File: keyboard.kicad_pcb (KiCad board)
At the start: 2 copper layers, 129.8 x 72.4 mm, 119 parts, among them P1 USB_B, P10 CONN_01X01, P2 CONN_02X03, P3 CONN_01X01, P4 CONN_01X01, P5 CONN_01X01, P6 CONN_01X01, P7 CONN_01X01, P8 CONN_01X01, P9 CONN_01X01, SW10 SW_PUSH, SW11 SW_PUSH, SW12 SW_PUSH, SW13 SW_PUSH, SW14 SW_PUSH, SW15 SW_PUSH, SW2 SW_PUSH, SW24 SW_PUSH, SW25 SW_PUSH, SW26 SW_PUSH, SW27 SW_PUSH, SW28 SW_PUSH, SW29 SW_PUSH, SW3 SW_PUSH, SW30 SW_PUSH, SW31 SW_PUSH, SW32 SW_PUSH, SW33 SW_PUSH, SW34 SW_PUSH, SW35 SW_PUSH, SW36 SW_PUSH, SW37 SW_PUSH, SW4 SW_PUSH, SW5 SW_PUSH, SW6 SW_PUSH, SW7 SW_PUSH, SW8 SW_PUSH, SW9 SW_PUSH, U1 ATmega32U4, X1 CRYSTAL_SMD

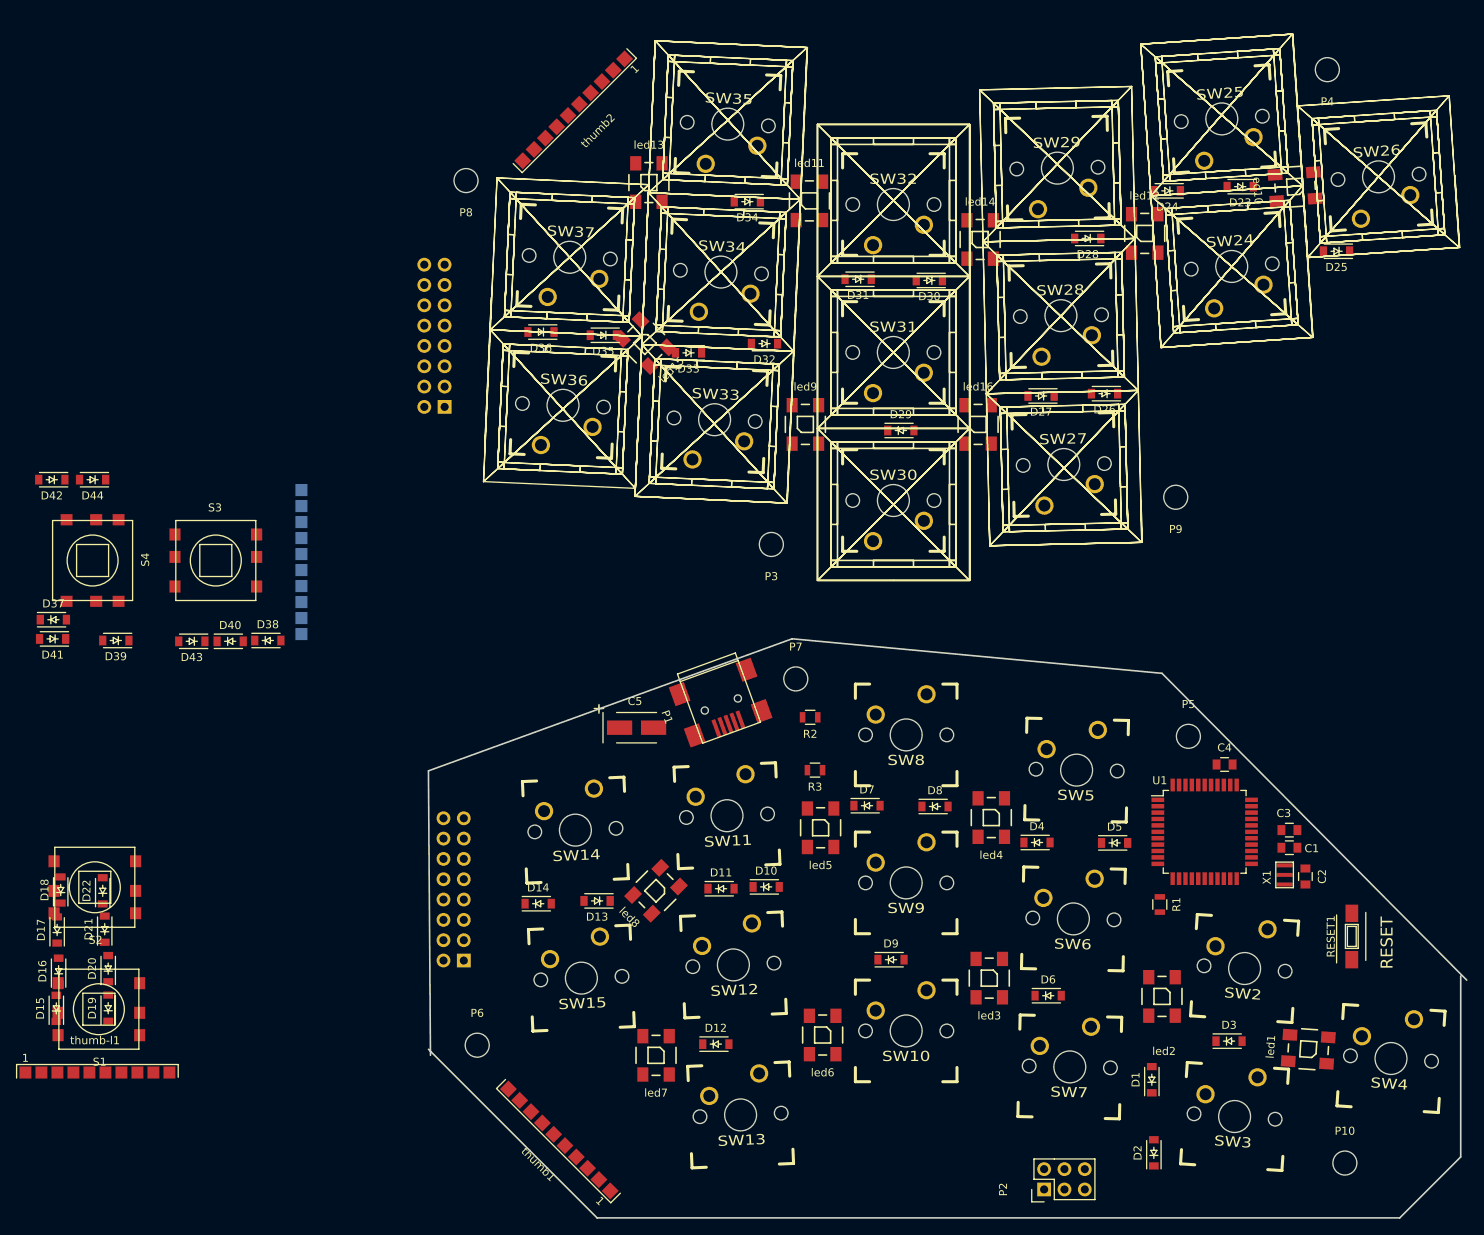
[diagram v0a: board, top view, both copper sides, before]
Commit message: nearly routed
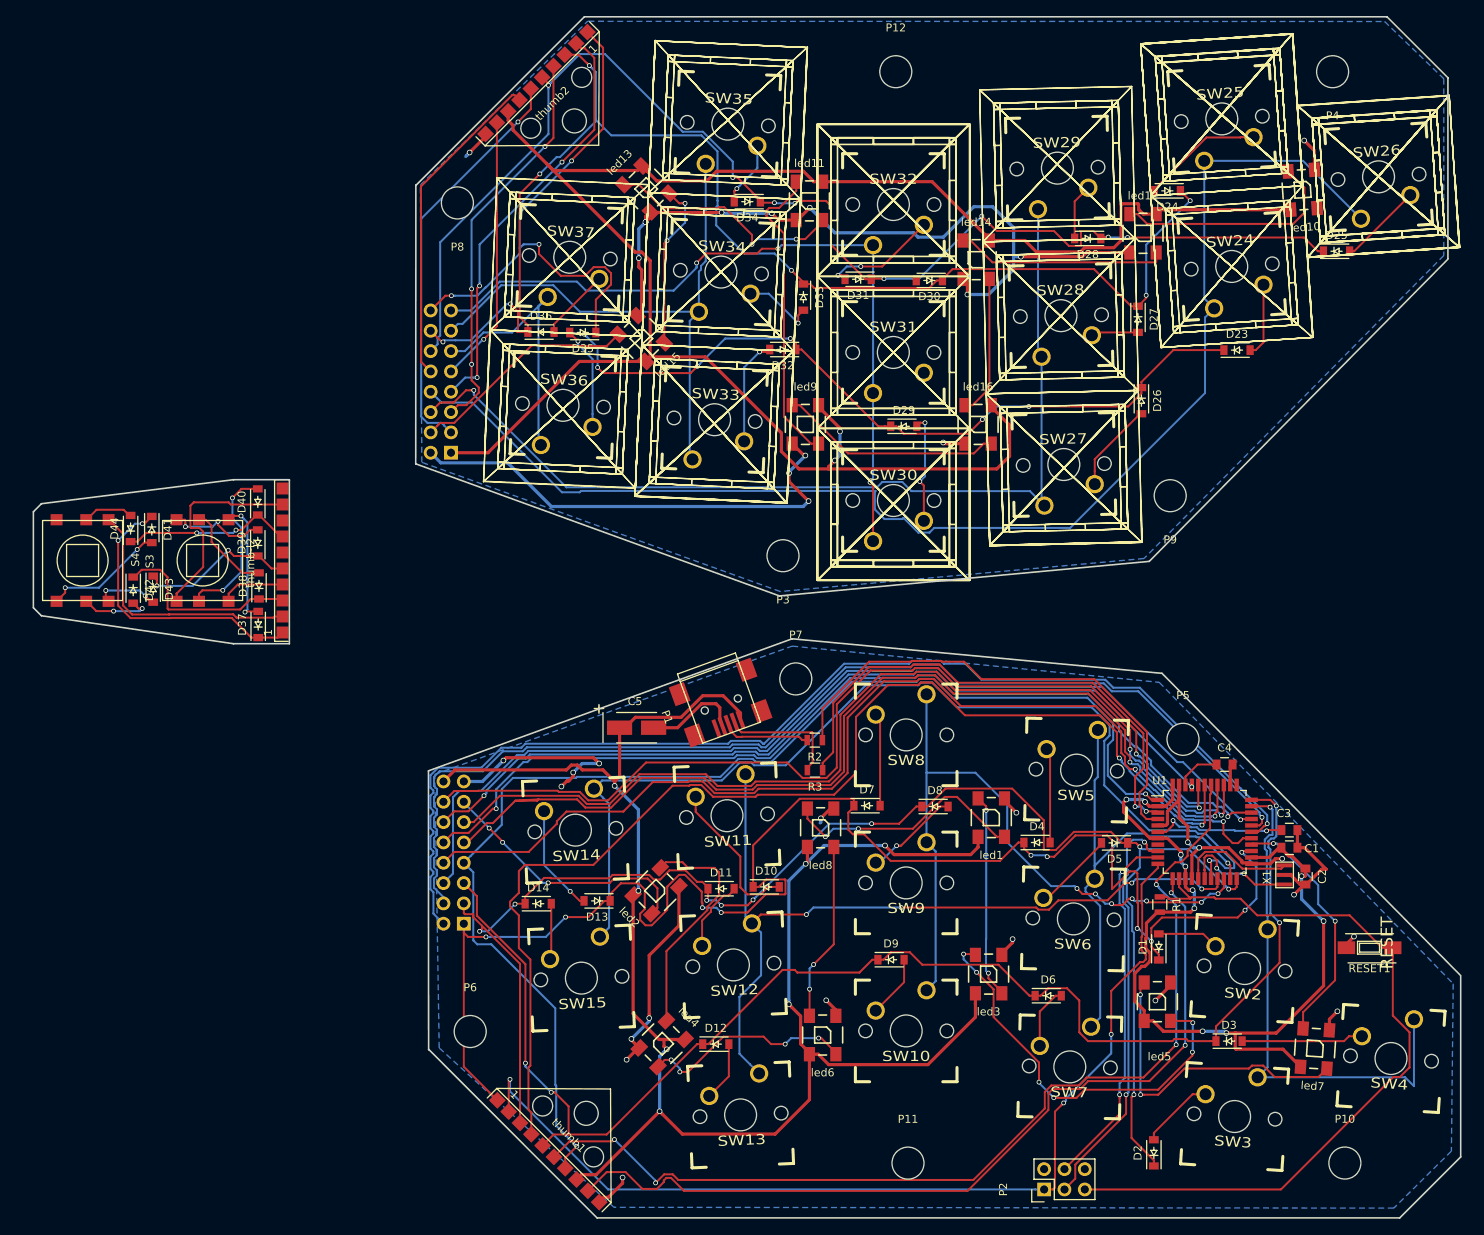
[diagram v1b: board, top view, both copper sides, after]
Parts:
- removed D15, D16, D17, D18, D19, D20, D21, D22: D, Diodes_SMD:SOD-123
- removed S1, S2: alps_4way, fp:alps 4way smt
- removed thumb-l1: CONN_02X05, fp:thumbpad connector
- added P11: CONN_01X01, Mounting_Holes:MountingHole_4mm, F.Cu at (148.8, 165.9)
- added P12: CONN_01X01, Mounting_Holes:MountingHole_4mm, F.Cu at (147.3, 29.5)
- P10, P3, P4, P5, P6, P7, P8, P9: footprint Mounting_Holes:MountingHole_3mm -> Mounting_Holes:MountingHole_4mm
- thumb-l2: moved to F.Cu
- moved conn1 64.6 mm to (93.3, 136.0)
- moved conn2 63.5 mm to (91.7, 77.1)
- moved D37 25.6 mm to (67.6, 98.6), turned to 90 degrees
- moved D39 21.5 mm to (67.5, 88.4), turned to 90 degrees
- moved D23 20.4 mm to (189.9, 64.3), turned to 0 degrees
- moved D41 18.5 mm to (54.3, 86.7), turned to 270 degrees
- moved thumb1 18.1 mm to (97.5, 158.1), turned to 315 degrees
- moved thumb-l2 18.0 mm to (70.7, 99.6), turned to 90 degrees
- moved D40 17.8 mm to (67.5, 83.3), turned to 90 degrees
- moved D42 17.1 mm to (52.0, 94.3), turned to 270 degrees
- moved D1 16.6 mm to (180.2, 138.9)
- moved D33 16.0 mm to (135.8, 57.7), turned to 270 degrees
- moved D27 15.4 mm to (177.6, 60.5), turned to 270 degrees
- moved D43 8.12 mm to (54.5, 94.2), turned to 270 degrees
- moved D44 7.73 mm to (51.6, 86.6), turned to 90 degrees
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- renumbered led4 to led1, led8 to led2, led7 to led4, led2 to led5, led1 to led7, led5 to led8
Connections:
- D1 pad 1: /left keys/row1 -> /right keys/row1
- D10 pad 1: /left keys/row1 -> /right keys/row1
- D11 pad 1: /left keys/row2 -> /right keys/row2
- D12 pad 1: /left keys/row3 -> /right keys/row3
- D13 pad 1: /left keys/row1 -> /right keys/row1
- D14 pad 1: /left keys/row2 -> /right keys/row2
- D2 pad 1: /left keys/row2 -> /right keys/row2
- D3 pad 1: /left keys/row3 -> /right keys/row3
- D37 pad 1: /left keys/row1 -> /left keys/thumb/row1
- D38 pad 1: /left keys/row2 -> /left keys/thumb/row2
- D39 pad 1: /left keys/row3 -> /left keys/thumb/row3
- D4 pad 1: /left keys/row1 -> /right keys/row1
- D40 pad 1: /left keys/row4 -> /left keys/thumb/row4
- D41 pad 1: /left keys/row1 -> /left keys/thumb/row1
- D42 pad 1: /left keys/row2 -> /left keys/thumb/row2
- D43 pad 1: /left keys/row3 -> /left keys/thumb/row3
- D44 pad 1: /left keys/row4 -> /left keys/thumb/row4
- D5 pad 1: /left keys/row2 -> /right keys/row2
- D6 pad 1: /left keys/row3 -> /right keys/row3
- D7 pad 1: /left keys/row1 -> /right keys/row1
- D8 pad 1: /left keys/row2 -> /right keys/row2
- D9 pad 1: /left keys/row3 -> /right keys/row3
- S3 pad 4: /left keys/col6 -> /left keys/thumb/col1
- S4 pad 4: /left keys/col7 -> /left keys/thumb/col2
- U1 pad 1: /left keys/row4 -> /right keys/row4
- U1 pad 22: /left keys/row2 -> /right keys/row2
- U1 pad 25: /left keys/row1 -> /right keys/row1
- U1 pad 27: /left keys/col6 -> /col6
- U1 pad 28: /left keys/col3 -> /col3
- U1 pad 29: /left keys/col4 -> /col4
- U1 pad 30: /left keys/col5 -> /col5
- U1 pad 31: /left keys/col7 -> /col7
- U1 pad 33: /left keys/row3 -> /right keys/row3
- U1 pad 36: /left keys/col2 -> /col2
- U1 pad 37: /left keys/col1 -> /col1
- U1 pad 40: /left keys/joy-y -> /l-joy-y
- U1 pad 41: /left keys/joy-x -> /l-joy-x
- conn1 pad 1: /left keys/row1 -> /right keys/row1
- conn1 pad 10: /left keys/col7 -> /col7
- conn1 pad 11: /left keys/col2 -> /col2
- conn1 pad 12: /left keys/joy-x -> /l-joy-x
- conn1 pad 13: /left keys/ws2812 -> /right keys/ws2812-out
- conn1 pad 14: /left keys/joy-y -> /l-joy-y
- conn1 pad 2: /left keys/col3 -> /col3
- conn1 pad 3: /left keys/row2 -> /right keys/row2
- conn1 pad 4: /left keys/col4 -> /col4
- conn1 pad 5: /left keys/row3 -> /right keys/row3
- conn1 pad 6: /left keys/col5 -> /col5
- conn1 pad 7: /left keys/row4 -> /right keys/row4
- conn1 pad 8: /left keys/col6 -> /col6
- conn1 pad 9: /left keys/col1 -> /col1
- conn2 pad 1: /left keys/row1 -> +5V
- conn2 pad 10: /left keys/col7 -> /left keys/row4
- conn2 pad 11: /left keys/col2 -> /left keys/col5
- conn2 pad 12: /left keys/joy-x -> /left keys/row3
- conn2 pad 13: /left keys/ws2812 -> /left keys/col4
- conn2 pad 14: /left keys/joy-y -> /left keys/row2
- conn2 pad 15: Earth -> /left keys/col3
- conn2 pad 16: +5V -> /left keys/row1
- conn2 pad 2: /left keys/col3 -> Earth
- conn2 pad 3: /left keys/row2 -> /left keys/joy-y
- conn2 pad 4: /left keys/col4 -> /left keys/ws2812
- conn2 pad 5: /left keys/row3 -> /left keys/joy-x
- conn2 pad 6: /left keys/col5 -> /left keys/col2
- conn2 pad 7: /left keys/row4 -> /left keys/col7
- conn2 pad 8: /left keys/col6 -> /left keys/col1
- conn2 pad 9: /left keys/col1 -> /left keys/col6
- led1 pad 2: Net-(led2-Pad4) -> Net-(led1-Pad2)
- led1 pad 4: Net-(led4-Pad4) -> Net-(led1-Pad4)
- led2 pad 2: Net-(led6-Pad4) -> /right keys/ws2812-out
- led2 pad 4: Net-(led1-Pad2) -> Net-(led2-Pad4)
- led4 pad 2: Net-(led5-Pad4) -> Net-(led2-Pad4)
- led4 pad 4: /right keys/ws2812 -> Net-(led4-Pad4)
- led5 pad 2: /left keys/ws2812 -> Net-(led3-Pad4)
- led5 pad 4: Net-(led2-Pad4) -> Net-(led5-Pad4)
- led7 pad 2: Net-(led1-Pad2) -> Net-(led5-Pad4)
- led7 pad 4: Net-(led1-Pad4) -> /right keys/ws2812
- led8 pad 2: Net-(led3-Pad4) -> Net-(led6-Pad4)
- led8 pad 4: Net-(led5-Pad4) -> Net-(led1-Pad2)
- thumb-l2 pad 1: /left keys/row1 -> /left keys/thumb/row1
- thumb-l2 pad 2: /left keys/col7 -> /left keys/thumb/col2
- thumb-l2 pad 3: /left keys/row2 -> /left keys/thumb/row2
- thumb-l2 pad 4: /left keys/joy-x -> (no net)
- thumb-l2 pad 5: /left keys/row3 -> /left keys/thumb/row3
- thumb-l2 pad 6: /left keys/joy-y -> (no net)
- thumb-l2 pad 7: /left keys/row4 -> /left keys/thumb/row4
- thumb-l2 pad 9: /left keys/col6 -> /left keys/thumb/col1
- thumb1 pad 1: /left keys/row1 -> /right keys/row1
- thumb1 pad 3: /left keys/row2 -> /right keys/row2
- thumb1 pad 5: /left keys/row3 -> /right keys/row3
- thumb1 pad 7: /left keys/row4 -> /right keys/row4
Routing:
- net +5V: track 0.00 -> 569.9 mm, vias 0 -> 19
- net Earth: track 0.00 -> 297.6 mm, vias 0 -> 33
- net /right keys/row1: track 0.00 -> 196.3 mm, vias 0 -> 10
- net /right keys/row2: track 0.00 -> 192.2 mm, vias 0 -> 9
- net /right keys/row3: track 0.00 -> 176.8 mm, vias 0 -> 4
- net /left keys/row1: track 0.00 -> 167.1 mm, vias 0 -> 9
- net /left keys/col1: track 0.00 -> 165.7 mm
- net /left keys/row3: track 0.00 -> 163.1 mm, vias 0 -> 8
- net /left keys/row2: track 0.00 -> 162.6 mm, vias 0 -> 7
- net /right keys/row4: track 0.00 -> 155.9 mm, vias 0 -> 2
- net /right keys/joy-x: track 0.00 -> 149.6 mm, vias 0 -> 2
- net /col3: track 0.00 -> 143.1 mm, vias 0 -> 1
- net /col4: track 0.00 -> 137.7 mm, vias 0 -> 1
- net /col6: track 0.00 -> 127.9 mm, vias 0 -> 2
- net /right keys/joy-y: track 0.00 -> 126.8 mm, vias 0 -> 4
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- added copper zone on B.Cu, net Earth
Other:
- board size 129.8 x 72.4 mm -> 178.4 x 150.1 mm
- net class power added: clearance 0.2, trace_width 0.4, via_dia 0.7, via_drill 0.5
- board text added: "check usb fp"
- board text removed: "10mm bolt with 6mm spacer"
- board text removed: "even holes are 22.63 mm away from bottom edge"
- board text removed: "right side"
- board text removed: "set back 1.205mm from edge of board insulator is 2mm above top of board"
